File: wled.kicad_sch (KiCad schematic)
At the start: 21 parts, among them J1 Audio pwr Selector, J2 Barrel_Jack_Switch, J3 Esp826, K1 FINDER-36.11, Q1 2N3904, U1 ESP32-DEVKIT-V1, U2 TSOP333xx

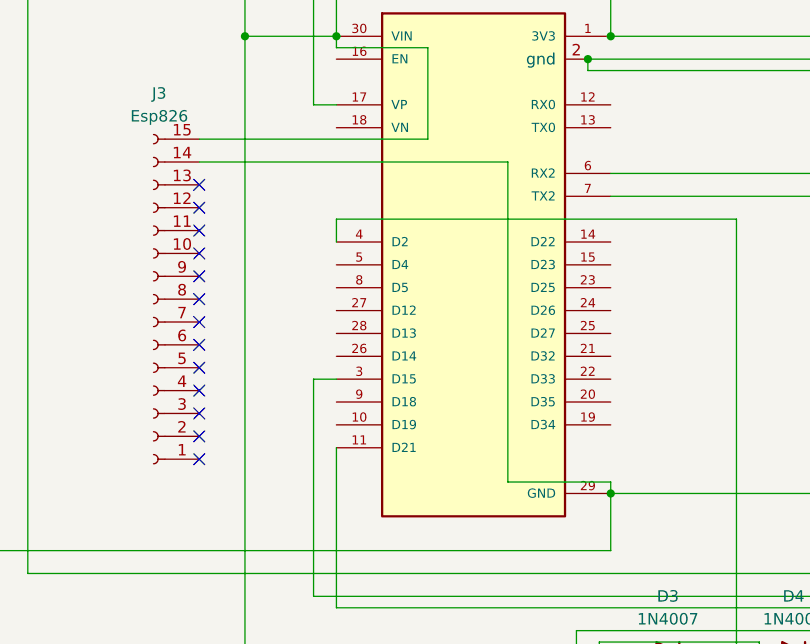
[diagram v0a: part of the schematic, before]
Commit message: t
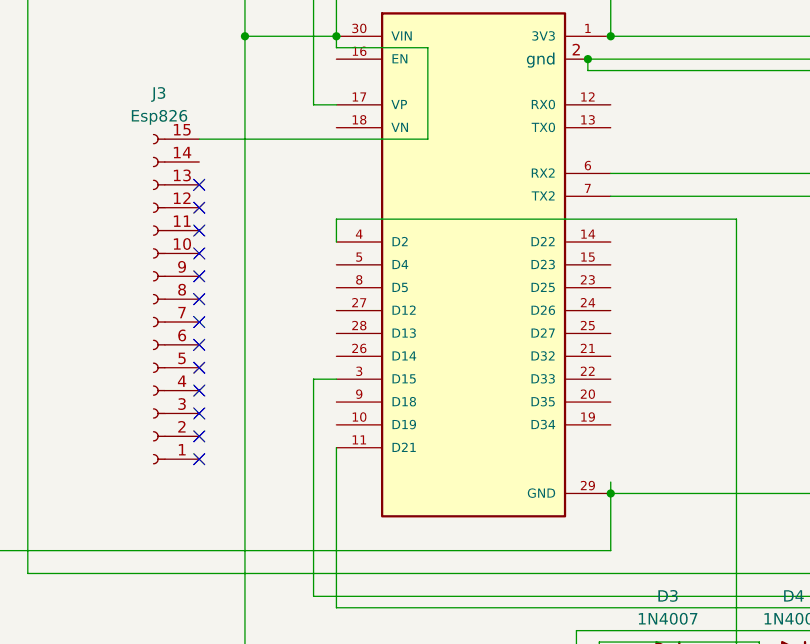
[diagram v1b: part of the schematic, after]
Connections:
- net at J2.2, J2.3, K1.1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: no longer J3.14 (Pin_14)
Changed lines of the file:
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@@
-	(wire
-		(pts
-			(xy 116.84 99.06) (xy 128.27 99.06)
-		)
-		(stroke
-			(width 0)
-			(type default)
-		)
-	)
 	(wire
 		(pts
@@
 	(wire
 		(pts
-			(xy 82.55 63.5) (xy 116.84 63.5)
-		)
-		(stroke
-			(width 0)
-			(type default)
-		)
-	)
-	(wire
-		(pts
 			(xy 55.88 40.64) (xy 55.88 43.18)
 		)
@@
 		)
 		(stroke
-			(width 0)
-			(type default)
-		)
-	)
-	(wire
-		(pts
-			(xy 116.84 63.5) (xy 116.84 99.06)
-		)
-		(stroke

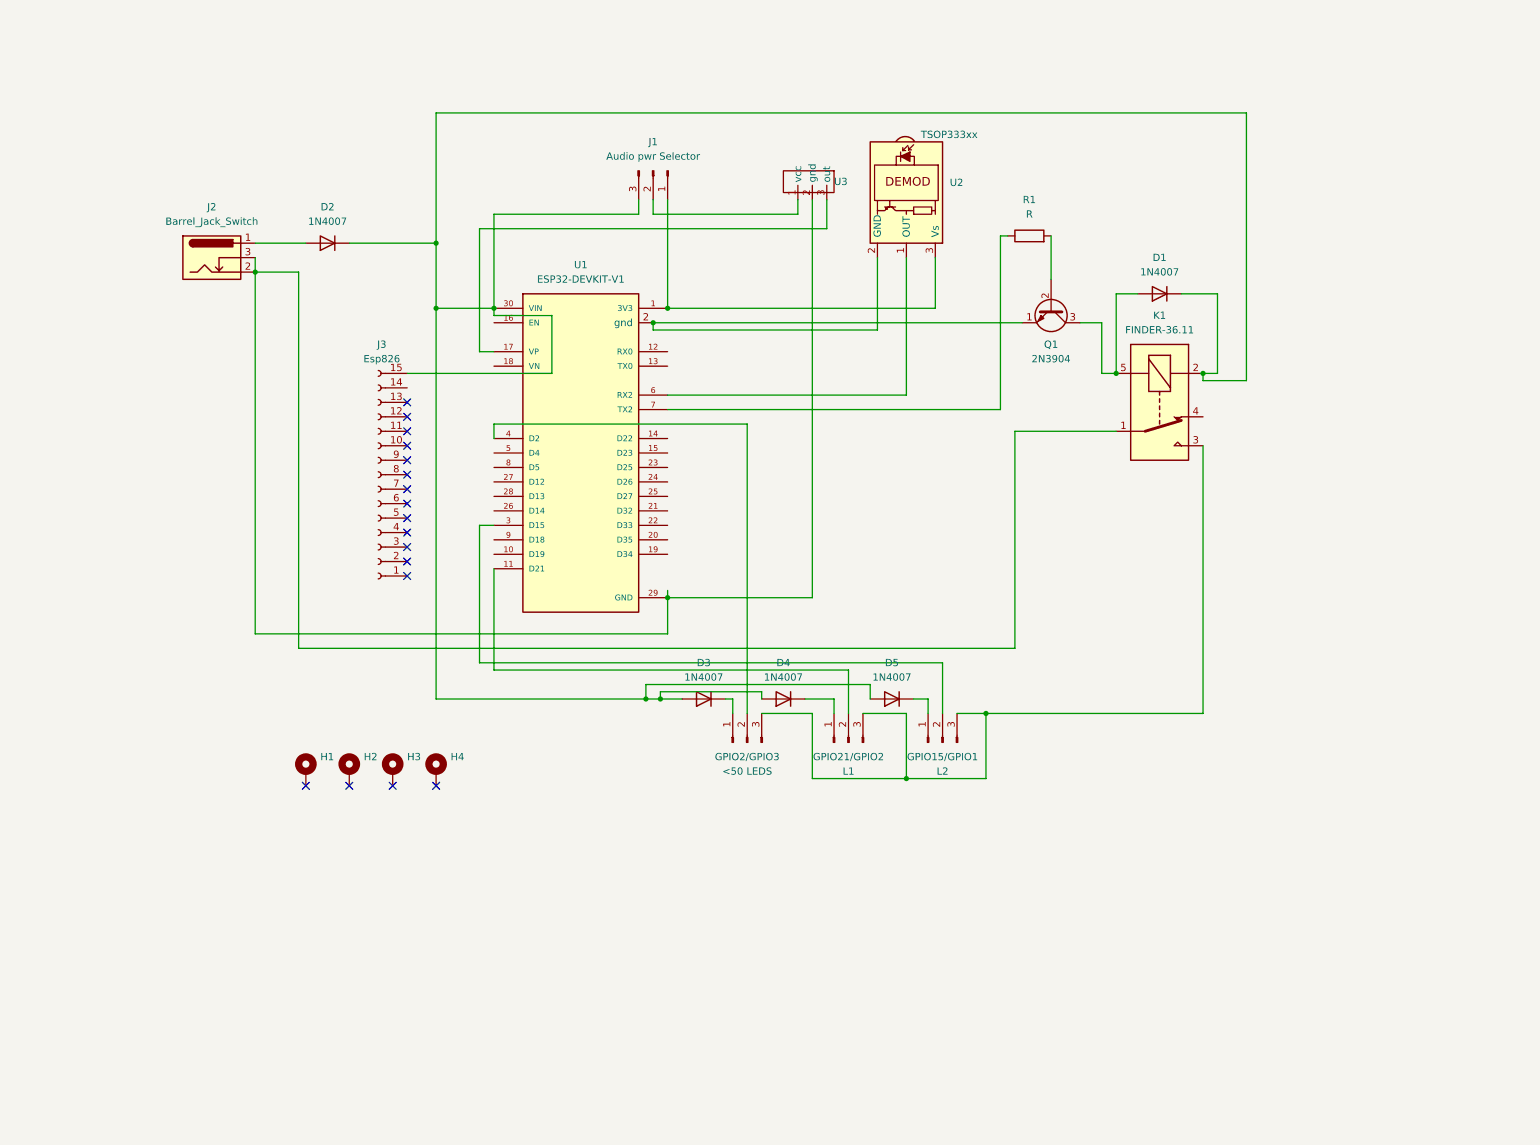
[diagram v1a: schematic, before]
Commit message: version-1.0 rev 2026-04-11
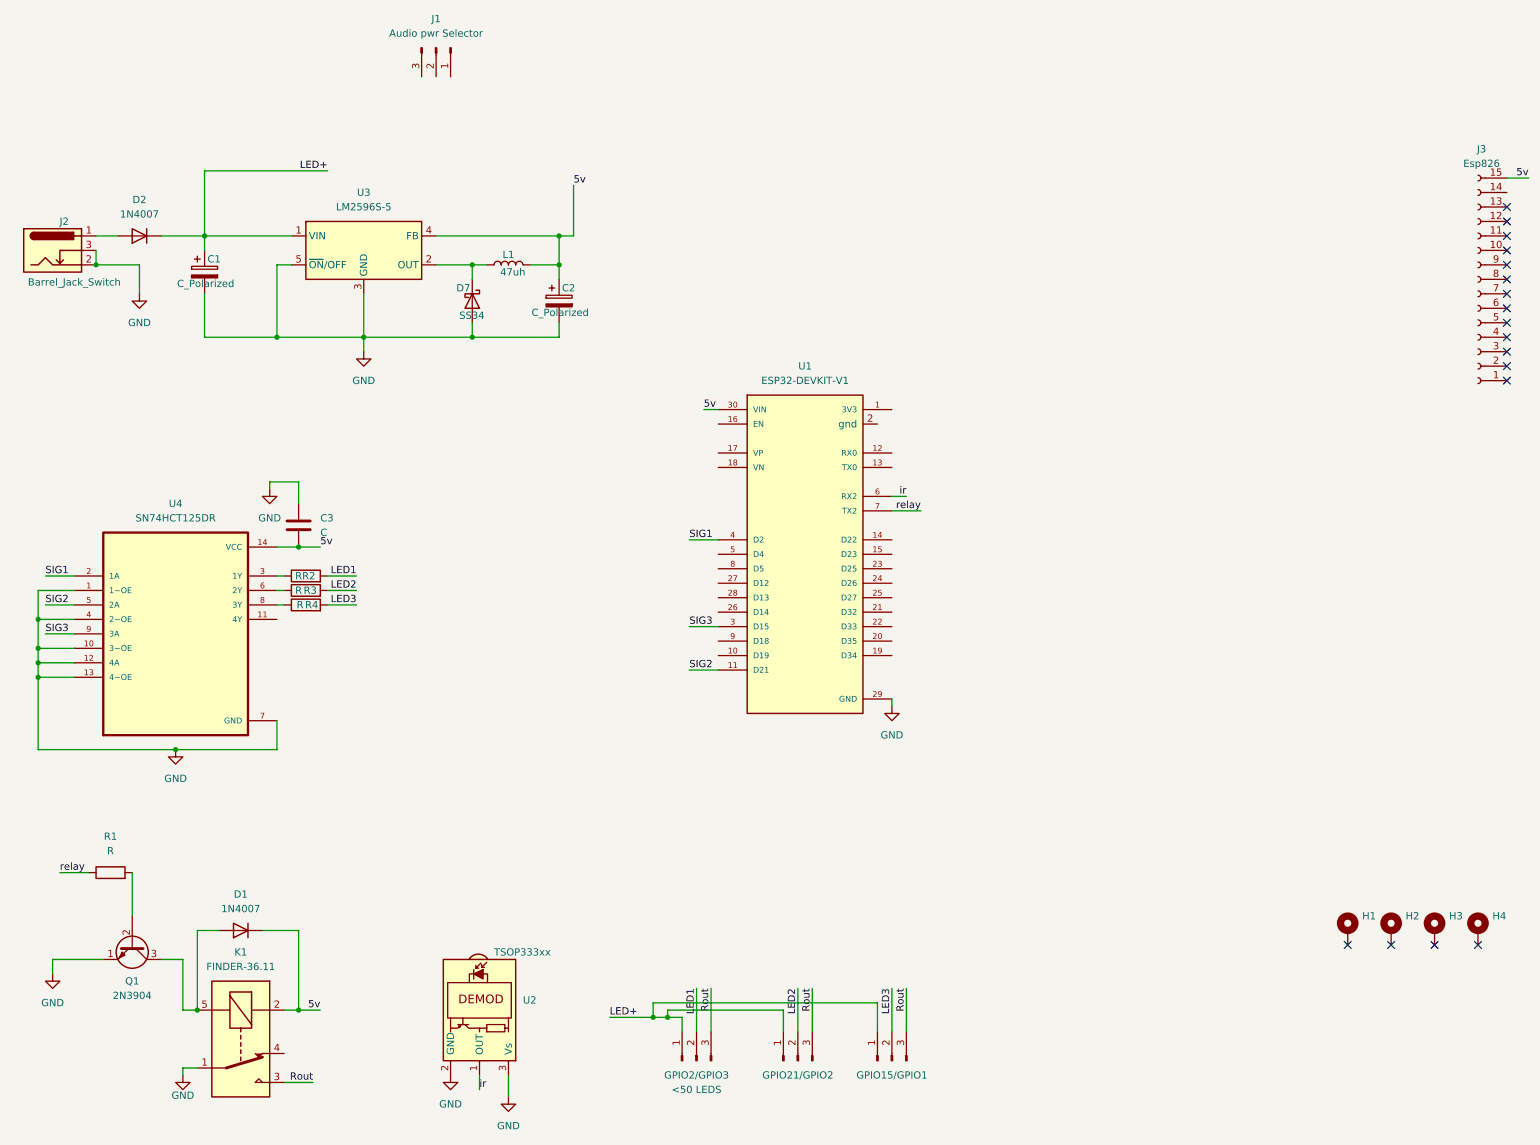
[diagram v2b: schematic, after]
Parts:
- removed D3, D4, D5: 1N4007, Diode_THT:D_DO-41_SOD81_P10.16mm_Horizontal, symbol Diode:1N4007
- removed U3: ~, sound sen:sound sens, symbol New_Library:sound_sensor
- added C1, C2: C_Polarized, Capacitor_THT:CP_Radial_D5.0mm_P2.50mm, symbol Device:C_Polarized
- added C3: C, symbol Device:C
- added D7: SS34, Diode_SMD:D_SMA, symbol Diode:SS34
- added L1: 47uh, Inductor_SMD:L_12x12mm_H6mm, symbol Device:L
- added R2, R3, R4: R, Resistor_THT:R_Axial_DIN0207_L6.3mm_D2.5mm_P5.08mm_Vertical, symbol Device:R
- added U3: LM2596S-5, Package_TO_SOT_SMD:TO-263-5_TabPin3, symbol Regulator_Switching:LM2596S-5
- added U4: SN74HCT125DR, SN74HCT125DR:SOIC127P600X175-14N, symbol SN74HCT125DR:SN74HCT125DR
- U1: footprint MODULE_ESP32_DEVKIT_V1:MODULE_ESP32_DEVKIT_V1 -> esp32_devkitV1:MODULE_ESP32_DEVKIT_V1
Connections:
- net relay: now reaches R1.1, U1.7 (TX2)
- net LED+: now reaches GPIO21/GPIO2.1 (Pin_1)
- net LED+: now also D2.1 (K), GPIO15/GPIO1.1 (Pin_1), GPIO2/GPIO3.1 (Pin_1), C1.1, U3.1 (VIN)
- net 5v: now reaches D1.1 (K), J3.15 (Pin_15), K1.2, U1.30 (VIN)
- net 5v: now also C2.1, C3.2, L1.2, U3.4 (FB), U4.14 (VCC); no longer D2.1 (K), J1.3 (Pin_3)
- net LED3: now reaches GPIO15/GPIO1.2 (Pin_2)
- net LED3: now also R4.2; no longer U1.3 (D15)
- net Rout: now reaches GPIO15/GPIO1.3 (Pin_3), GPIO2/GPIO3.3 (Pin_3), GPIO21/GPIO2.3 (Pin_3), K1.3
- net ir: now reaches U1.6 (RX2), U2.1 (OUT)
- net GND: now reaches Q1.1 (E), U2.2 (GND)
- net GND: now also J2.2, J2.3, K1.1, U1.29 (GND), U2.3 (Vs), C1.2, C2.2, C3.1, D7.2 (A), U3.3 (GND), U3.5 (~{ON}/OFF), U4.1 (1~OE), U4.10 (3~OE), U4.12 (4A), U4.13 (4~OE), U4.4 (2~OE), U4.7 (GND); no longer U1.2 (gnd)
- net LED2: now reaches GPIO21/GPIO2.2 (Pin_2)
- net LED2: now also R3.2; no longer U1.11 (D21)
- net LED1: now reaches GPIO2/GPIO3.2 (Pin_2)
- net LED1: now also R2.2; no longer U1.4 (D2)
- new net: R2.1, U4.3 (1Y)
- new net: D7.1 (K), L1.1, U3.2 (OUT)
- new net: R4.1, U4.8 (3Y)
- new net: R3.1, U4.6 (2Y)
- new net SIG1: U1.4 (D2), U4.2 (1A)
- new net SIG2: U1.11 (D21), U4.5 (2A)
- new net SIG3: U1.3 (D15), U4.9 (3A)
- now unconnected: J1.1 (Pin_1), U1.1 (3V3)
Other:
- moved on the sheet: D1, D2, GPIO15/GPIO1, GPIO2/GPIO3, GPIO21/GPIO2, H1, H2, H3, H4, J1, J2, J3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

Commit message: New wled controller -smd with S3 Wroom-1 chip
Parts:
- removed C1, C2: C_Polarized, Capacitor_THT:CP_Radial_D5.0mm_P2.50mm, symbol Device:C_Polarized
- removed D1, D2: 1N4007, Diode_THT:D_DO-41_SOD81_P10.16mm_Horizontal, symbol Diode:1N4007
- removed D7: SS34, Diode_SMD:D_SMA, symbol Diode:SS34
- removed GPIO15/GPIO1: L2, Connector_Wire:SolderWire-0.127sqmm_1x03_P3.7mm_D0.48mm_OD1mm_Relief, symbol Connector:Conn_01x03_Pin
- removed J1: Audio pwr Selector, Connector_PinHeader_2.54mm:PinHeader_1x03_P2.54mm_Horizontal, symbol Connector:Conn_01x03_Pin
- removed J2: Barrel_Jack_Switch, Connector_BarrelJack:BarrelJack_CUI_PJ-102AH_Horizontal, symbol Connector:Barrel_Jack_Switch
- removed J3: Esp826, Connector_PinHeader_2.54mm:PinHeader_1x15_P2.54mm_Vertical, symbol Connector:Conn_01x15_Socket
- removed K1: FINDER-36.11, Relay_THT:Relay_SPDT_Omron-G5LE-1, symbol Relay:FINDER-36.11
- removed L1: 47uh, Inductor_SMD:L_12x12mm_H6mm, symbol Device:L
- removed Q1: 2N3904, Package_TO_SOT_THT:TO-92_Inline, symbol Transistor_BJT:2N3904
- removed U1: ESP32-DEVKIT-V1, esp32_devkitV1:MODULE_ESP32_DEVKIT_V1, symbol ESP32-DEVKIT-V1:ESP32-DEVKIT-V1
- removed U2: TSOP333xx, OptoDevice:Vishay_MINIMOLD-3Pin, symbol Interface_Optical:TSOP333xx
- removed U3: LM2596S-5, Package_TO_SOT_SMD:TO-263-5_TabPin3, symbol Regulator_Switching:LM2596S-5
- added 100uf1: C_Tantalum, Capacitor_Tantalum_SMD:CP_EIA-3216-10_Kemet-I, symbol Device:C_Polarized
- added C1: 1uf, Capacitor_SMD:C_1206_3216Metric_Pad1.33x1.80mm_HandSolder, symbol Device:C
- added C10, C11, C4, C6: 100nF, Capacitor_SMD:C_1206_3216Metric_Pad1.33x1.80mm_HandSolder, symbol Device:C
- added C13: 0.1uF, Capacitor_SMD:C_1206_3216Metric_Pad1.33x1.80mm_HandSolder, symbol Device:C
- added C2, C8: 0u1f, Capacitor_SMD:C_1206_3216Metric_Pad1.33x1.80mm_HandSolder, symbol Device:C
- added C5, C9: C_Polarized_Small, Capacitor_THT:CP_Radial_D8.0mm_P3.50mm, symbol PCM_SparkFun-Capacitor:C_Polarized_Small
- added C7: 100nf, Capacitor_SMD:C_1206_3216Metric_Pad1.33x1.80mm_HandSolder, symbol Device:C
- added CP1, CP2: 10uf, Capacitor_SMD:C_1206_3216Metric_Pad1.33x1.80mm_HandSolder, symbol Device:C_Polarized
- added D3: D_Schottky, Resistor_SMD:R_0805_2012Metric_Pad1.20x1.40mm_HandSolder, symbol Device:D_Schottky
- added D4: SS34, Diode_SMD:D_SMA, symbol Diode:SS34
- added D6: ESP-PWR, Capacitor_SMD:C_1206_3216Metric_Pad1.33x1.80mm_HandSolder, symbol Device:LED
- added DZ2: 1N5240B, PCM_Diode_THT_AKL:D_DO-35_SOD27_P7.62mm_Horizontal_Zener, symbol PCM_Diode_Zener_AKL:1N5240B
- added J1: Screw_Terminal_01x02, Connector_Phoenix_MC_HighVoltage:PhoenixContact_MC_1,5_2-G-5.08_1x02_P5.08mm_Horizontal, symbol Connector:Screw_Terminal_01x02
- added J2: GPIO, TerminalBlock:TerminalBlock_Xinya_XY308-2.54-2P_1x02_P2.54mm_Horizontal, symbol Connector:Screw_Terminal_01x02
- added J3: JST_2mm_3, PCM_SparkFun-Connector:JST_1x03_P2.0mm_Horizontal_PTH, symbol PCM_SparkFun-Connector:Conn_01x03_JST_P2.0mm_Horizontal_PTH
- added J4: USB_C_Receptacle_USB2.0_16P, Connector_USB:USB_C_Receptacle_GCT_USB4105-xx-A_16P_TopMnt_Horizontal, symbol Connector:USB_C_Receptacle_USB2.0_16P
- added L2: L, Inductor_SMD:L_10.4x10.4_H4.8, symbol Device:L
- added MIC1: Conn_01x06_Pin, Connector_JST:JST_EH_B6B-EH-A_1x06_P2.50mm_Vertical, symbol Connector:Conn_01x06_Pin
- added MK1: INMP441ACEZ-R7, INMP441ACEZ-R7:MIC_INMP441ACEZ-R7, symbol INMP441:INMP441ACEZ-R7
- added PwrSelector1: Conn_01x03_Pin, Connector_PinHeader_2.54mm:PinHeader_1x03_P2.54mm_Horizontal, symbol Connector:Conn_01x03_Pin
- added Q2: AUIRF4905, PCM_Package_TO_SOT_THT_AKL:TO-220-3_Horizontal_TabDown_GDS, symbol PCM_Transistor_MOSFET_AKL:AUIRF4905
- added R14, R5: 100k, Resistor_SMD:R_1206_3216Metric_Pad1.30x1.75mm_HandSolder, symbol Device:R
- added R16: 1k, Resistor_SMD:R_1206_3216Metric_Pad1.30x1.75mm_HandSolder, symbol Device:R
- added R23, R24: 10k, Resistor_SMD:R_1206_3216Metric_Pad1.30x1.75mm_HandSolder, symbol Device:R
- added R7, R8: 5.1k, Resistor_SMD:R_1206_3216Metric_Pad1.30x1.75mm_HandSolder, symbol Device:R
- added SW1, SW2: SW_Push, Button_Switch_THT:SW_PUSH_6mm_H13mm, symbol Switch:SW_Push
- added TP1, TP2, TP3, TP4: TestPoint, PCM_SparkFun-Connector:TestPoint-1.0mm, symbol Connector:TestPoint
- added U1: LM2596S-ADJ, Package_TO_SOT_SMD:TO-263-5_TabPin3, symbol Regulator_Switching:LM2596S-ADJ
- added U3: ESP32-S3-WROOM-1, RF_Module:ESP32-S3-WROOM-1, symbol RF_Module:ESP32-S3-WROOM-1
- added U5: AMS1117-3.3, Package_TO_SOT_SMD:SOT-223-3_TabPin2, symbol Regulator_Linear:AMS1117-3.3
- C3: footprint (none) -> Capacitor_SMD:C_1206_3216Metric_Pad1.33x1.80mm_HandSolder
- GPIO2/GPIO3, GPIO21/GPIO2: footprint Connector_Wire:SolderWire-0.127sqmm_1x03_P3.7mm_D0.48mm_OD1mm_Relief -> Connector_Phoenix_MC_HighVoltage:PhoenixContact_MC_1,5_3-G-5.08_1x03_P5.08mm_Horizontal
- R1: value R -> 100k; footprint Resistor_THT:R_Axial_DIN0207_L6.3mm_D2.5mm_P5.08mm_Vertical -> Resistor_SMD:R_1206_3216Metric_Pad1.30x1.75mm_HandSolder
- R2, R3: footprint Resistor_THT:R_Axial_DIN0207_L6.3mm_D2.5mm_P5.08mm_Vertical -> Resistor_SMD:R_1206_3216Metric_Pad1.30x1.75mm_HandSolder
- R4: value R -> 10k; footprint Resistor_THT:R_Axial_DIN0207_L6.3mm_D2.5mm_P5.08mm_Vertical -> Resistor_SMD:R_1206_3216Metric_Pad1.30x1.75mm_HandSolder
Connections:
- net LED+ is gone; now on net GND: GPIO2/GPIO3.1 (Pin_1), GPIO21/GPIO2.1 (Pin_1)
- net SIG3 is gone; now on net GND: U4.9 (3A)
- net relay is gone; now on net GND: R1.1
- net GND: now also 100uf1.2, C1.1, C10.1, C11.1, C13.1, C2.1, C4.1, C5.2, C6.1, C7.1, C8.1, C9.2, CP1.2, CP2.2, D4.2 (A), D6.1 (K), J1.2 (Pin_2), J2.2 (Pin_2), J3.3, J4.A1 (GND), J4.A12 (GND), J4.B1 (GND), J4.B12 (GND), J4.S1 (SHIELD), MIC1.2 (Pin_2), MK1.5 (GND), MK1.6 (GND), MK1.9 (GND), R14.1, R5.2, R7.2, R8.2, SW1.1, SW2.1, U1.3 (GND), U1.5 (~{ON}/OFF), U3.1 (GND), U3.40 (GND), U3.41 (GND), U5.1 (GND)
- net SIG1: now also U3.18 (IO10)
- net SIG2: now also U3.17 (IO9)
- net ir: now also J3.2, U3.25 (IO48)
- net SD: now reaches R1.2
- net SD: now also MIC1.5 (Pin_5), MK1.2 (SD), U3.4 (IO4)
- net at U4.8 (3Y): no longer R4.1
- net 5v renamed 5V
- net 5V: now also C10.2, C6.2, C9.1, CP1.1, D3.1 (K), L2.2, PwrSelector1.3 (Pin_3), TP2.1, U1.4 (FB), U5.3 (VI)
- net LED3 renamed ESP32_EN
- net ESP32_EN: now also C1.2, C8.2, R24.2, SW1.2, TP3.1, U3.3 (EN)
- net Rout renamed Vled
- net Vled: now also PwrSelector1.2 (Pin_2)
- new net: J4.A5 (CC1), R7.1
- new net: D3.2 (A), J4.A4 (VBUS), J4.A9 (VBUS), J4.B4 (VBUS), J4.B9 (VBUS)
- new net: DZ2.2 (A), Q2.1 (G), R14.2
- new net: J1.1 (Pin_1), Q2.2 (D)
- new net: D4.1 (K), L2.1, U1.2 (OUT)
- new net: D6.2 (A), R16.1
- new net: J4.B5 (CC2), R8.1
- new net 12V: C4.2, C5.1, DZ2.1 (K), PwrSelector1.1 (Pin_1), Q2.3 (S), U1.1 (VIN)
- new net 3V3: 100uf1.1, C11.2, C13.2, C7.2, CP2.1, J3.1, MIC1.1 (Pin_1), MK1.7 (VDD), R16.2, R23.1, R24.1, R4.1, TP1.1, U3.2 (3V3), U5.2 (VO)
- new net D+: J4.A6 (D+), J4.B6 (D+), U3.14 (USB_D+)
- new net D-: J4.A7 (D-), J4.B7 (D-), U3.13 (USB_D-)
- new net ESP32_IO0: C2.2, R23.2, SW2.2, TP4.1, U3.27 (IO0)
- new net GPIO: J2.1 (Pin_1), U3.24 (IO47)
- new net L/R: MIC1.3 (Pin_3), MK1.4 (L/R), R5.1
- new net SCK: MIC1.6 (Pin_6), MK1.1 (SCK), U3.6 (IO6)
- new net WS: MIC1.4 (Pin_4), MK1.3 (WS), U3.5 (IO5)
- no-connect marks 17 -> 10
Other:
- moved on the sheet: C3, GPIO2/GPIO3, GPIO21/GPIO2, H1, H2, H3, H4, R2, R3, U4
